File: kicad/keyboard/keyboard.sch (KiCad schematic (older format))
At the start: 132 parts, among them K0 KEYSW, K1 KEYSW, K10 KEYSW, K11 KEYSW, K12 KEYSW, K13 KEYSW, K14 KEYSW, K15 KEYSW, K16 KEYSW, K17 KEYSW, K18 KEYSW, K19 KEYSW, K2 KEYSW, K20 KEYSW, K21 KEYSW, K22 KEYSW, K23 KEYSW, K24 KEYSW, K25 KEYSW, K26 KEYSW, K27 KEYSW, K28 KEYSW, K29 KEYSW, K3 KEYSW, K30 KEYSW, K31 KEYSW, K32 KEYSW, K33 KEYSW, K34 KEYSW, K35 KEYSW, K36 KEYSW, K37 KEYSW, K38 KEYSW, K39 KEYSW, K4 KEYSW, K40 KEYSW, K41 KEYSW, K42 KEYSW, K43 KEYSW, K44 KEYSW, K45 KEYSW, K46 KEYSW, K47 KEYSW, K48 KEYSW, K49 KEYSW, K5 KEYSW, K50 KEYSW, K51 KEYSW, K52 KEYSW, K53 KEYSW, K54 KEYSW, K55 KEYSW, K56 KEYSW, K57 KEYSW, K58 KEYSW, K59 KEYSW, K6 KEYSW, K60 KEYSW, K61 KEYSW, K62 KEYSW, K63 KEYSW, K64 KEYSW, K65 KEYSW, K7 KEYSW, K9 KEYSW, U0 ProMicro, U1 74HC595

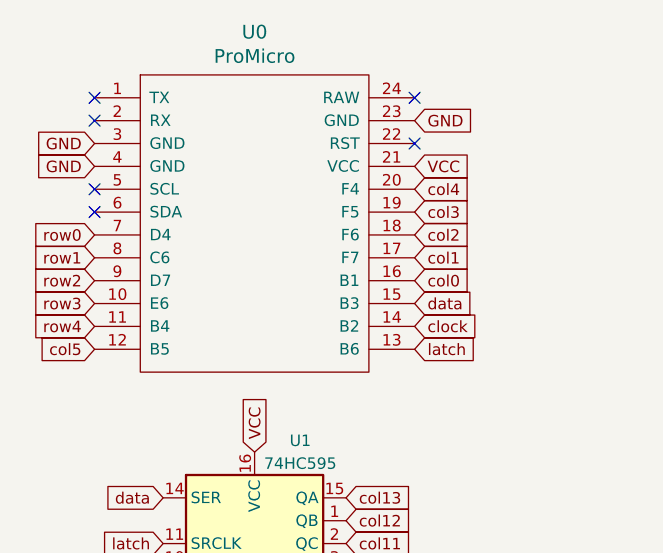
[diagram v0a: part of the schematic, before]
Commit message: flipped arduino to other side
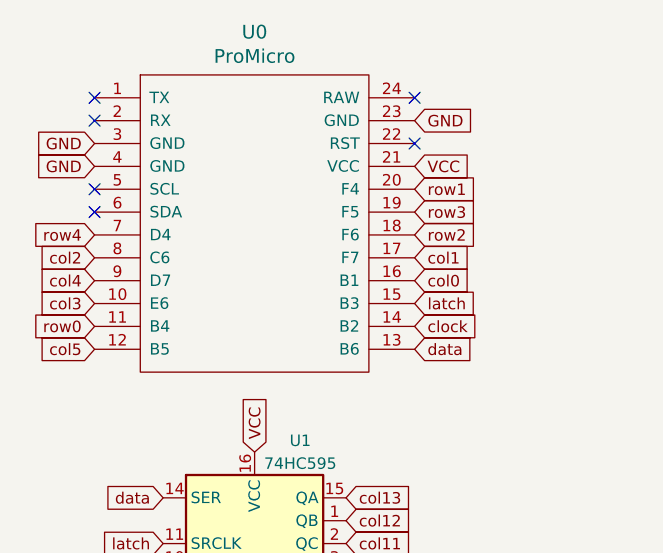
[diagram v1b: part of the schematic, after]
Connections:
- net col2: now also U0.8 (C6); no longer U0.18 (F6)
- net col3: now also U0.10 (E6); no longer U0.19 (F5)
- net col4: now also U0.9 (D7); no longer U0.20 (F4)
- net data: now also U0.13 (B6); no longer U0.15 (B3)
- net latch: now also U0.15 (B3); no longer U0.13 (B6)
- net row0: now also U0.11 (B4); no longer U0.7 (D4)
- net row1: now also U0.20 (F4); no longer U0.8 (C6)
- net row2: now also U0.18 (F6); no longer U0.9 (D7)
- net row3: now also U0.19 (F5); no longer U0.10 (E6)
- net row4: now also U0.7 (D4); no longer U0.11 (B4)
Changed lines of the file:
@@
 	750  5650 1050 5650
 Connection ~ 1550 5650
-Text GLabel 2150 2000 2    50   Input ~ 0
-latch
 Text GLabel 2150 1900 2    50   Input ~ 0
 clock
-Text GLabel 2150 1800 2    50   Input ~ 0
+Text GLabel 2150 2000 2    50   Input ~ 0
 data
 Text GLabel 2150 1200 2    50   Input ~ 0
@@
 Text GLabel 3200 4450 1    50   Input ~ 0
 col4
+Text GLabel 750  1900 0    50   Input ~ 0
+row0
 Text GLabel 750  1500 0    50   Input ~ 0
-row0
-Text GLabel 750  1900 0    50   Input ~ 0
 row4
-Text GLabel 750  1600 0    50   Input ~ 0
+Text GLabel 2150 1300 2    50   Input ~ 0
 row1
-Text GLabel 750  1700 0    50   Input ~ 0
+Text GLabel 2150 1500 2    50   Input ~ 0
 row2
-Text GLabel 750  1800 0    50   Input ~ 0
+Text GLabel 2150 1400 2    50   Input ~ 0
 row3
 Text GLabel 750  5650 0    50   Input ~ 0
@@
 Text GLabel 750  2000 0    50   Input ~ 0
 col5
-Text GLabel 2150 1300 2    50   Input ~ 0
+Text GLabel 750  1700 0    50   Input ~ 0
 col4
-Text GLabel 2150 1400 2    50   Input ~ 0
+Text GLabel 750  1800 0    50   Input ~ 0
 col3
 Text GLabel 1850 3350 2    50   Input ~ 0
@@
 Text GLabel 2150 1600 2    50   Input ~ 0
 col1
-Text GLabel 2150 1500 2    50   Input ~ 0
+Text GLabel 750  1600 0    50   Input ~ 0
 col2
 Wire Wire Line
@@
 col10
 NoConn ~ 1850 3550
+Text GLabel 2150 1800 2    50   Input ~ 0
+latch
 $EndSCHEMATC
